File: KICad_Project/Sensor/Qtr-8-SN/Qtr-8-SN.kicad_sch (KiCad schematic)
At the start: 37 parts, among them Q1 NMOS

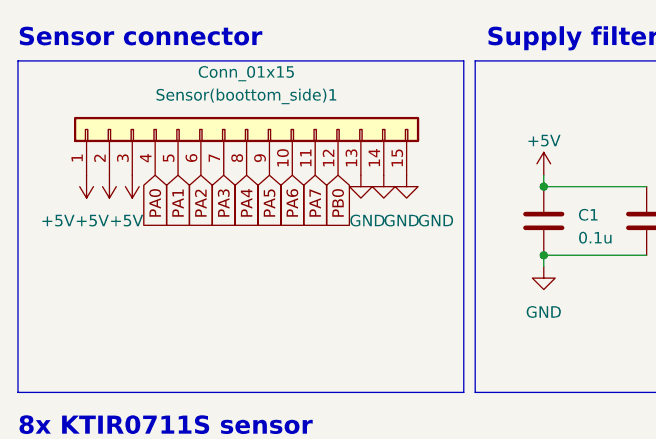
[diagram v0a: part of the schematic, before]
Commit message: 0.3
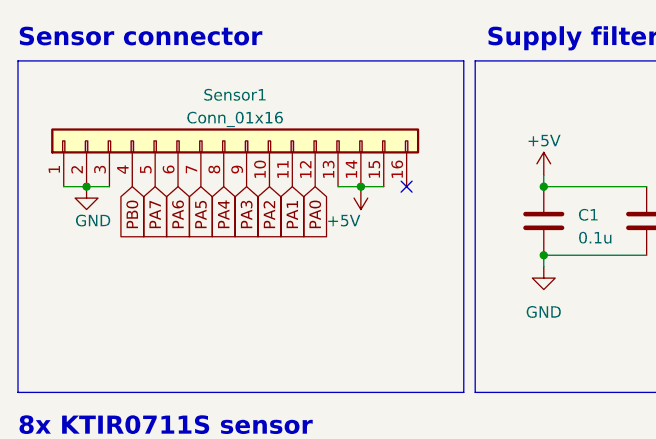
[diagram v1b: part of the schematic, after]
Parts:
- removed Sensor(boottom_side)1: Conn_01x15, Connector_FFC-FPC:Molex_200528-0150_1x15-1MP_P1.00mm_Horizontal, symbol Connector_Generic:Conn_01x15
- added Sensor1: Conn_01x16, Connector_FFC-FPC:Molex_200528-0160_1x16-1MP_P1.00mm_Horizontal, symbol Connector_Generic:Conn_01x16
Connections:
- net +5V: now also Sensor1.13 (Pin_13), Sensor1.14 (Pin_14), Sensor1.15 (Pin_15)
- net GND: now also Sensor1.1 (Pin_1), Sensor1.2 (Pin_2), Sensor1.3 (Pin_3)
- net PA0: now also Sensor1.12 (Pin_12)
- net PA1: now also Sensor1.11 (Pin_11)
- net PA2: now also Sensor1.10 (Pin_10)
- net PA3: now also Sensor1.9 (Pin_9)
- net PA4: now also Sensor1.8 (Pin_8)
- net PA5: now also Sensor1.7 (Pin_7)
- net PA6: now also Sensor1.6 (Pin_6)
- net PA7: now also Sensor1.5 (Pin_5)
- net PB0: now also Sensor1.4 (Pin_4)
- no-connect marks 4 -> 5
